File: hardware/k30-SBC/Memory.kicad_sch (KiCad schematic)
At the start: 3 parts, among them U14 AS6C8016, U15 AS6C8016, U16 AM29F040

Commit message: Upgraded project formats to kicad 6.0
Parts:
- U14, U15: symbol ComputieParts:AS6C8016 -> Computie_Memory:AS6C8016
- U16: symbol ComputieParts:AM29F040 -> Computie_Memory:AM29F040
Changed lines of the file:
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@@
     )
   )
-  (symbol (lib_id "ComputieParts:AS6C8016") (at 76.2 58.42 0) (unit 1)
+  (symbol (lib_id "Computie_Memory:AS6C8016") (at 76.2 58.42 0) (unit 1)
     (in_bom yes) (on_board yes)
     (property "Reference" "U14" (id 0) (at 76.2 25.8826 0))
@@
     (pin "9")
   )
-  (symbol (lib_id "ComputieParts:AS6C8016") (at 76.2 138.43 0) (unit 1)
+  (symbol (lib_id "Computie_Memory:AS6C8016") (at 76.2 138.43 0) (unit 1)
     (in_bom yes) (on_board yes)
     (property "Reference" "U15" (id 0) (at 76.2 105.8926 0))
@@
     (pin "1")
   )
-  (symbol (lib_id "ComputieParts:AM29F040") (at 176.53 55.88 0) (unit 1)
+  (symbol (lib_id "Computie_Memory:AM29F040") (at 176.53 55.88 0) (unit 1)
     (in_bom yes) (on_board yes)
     (property "Reference" "U16" (id 0) (at 176.53 25.8826 0))

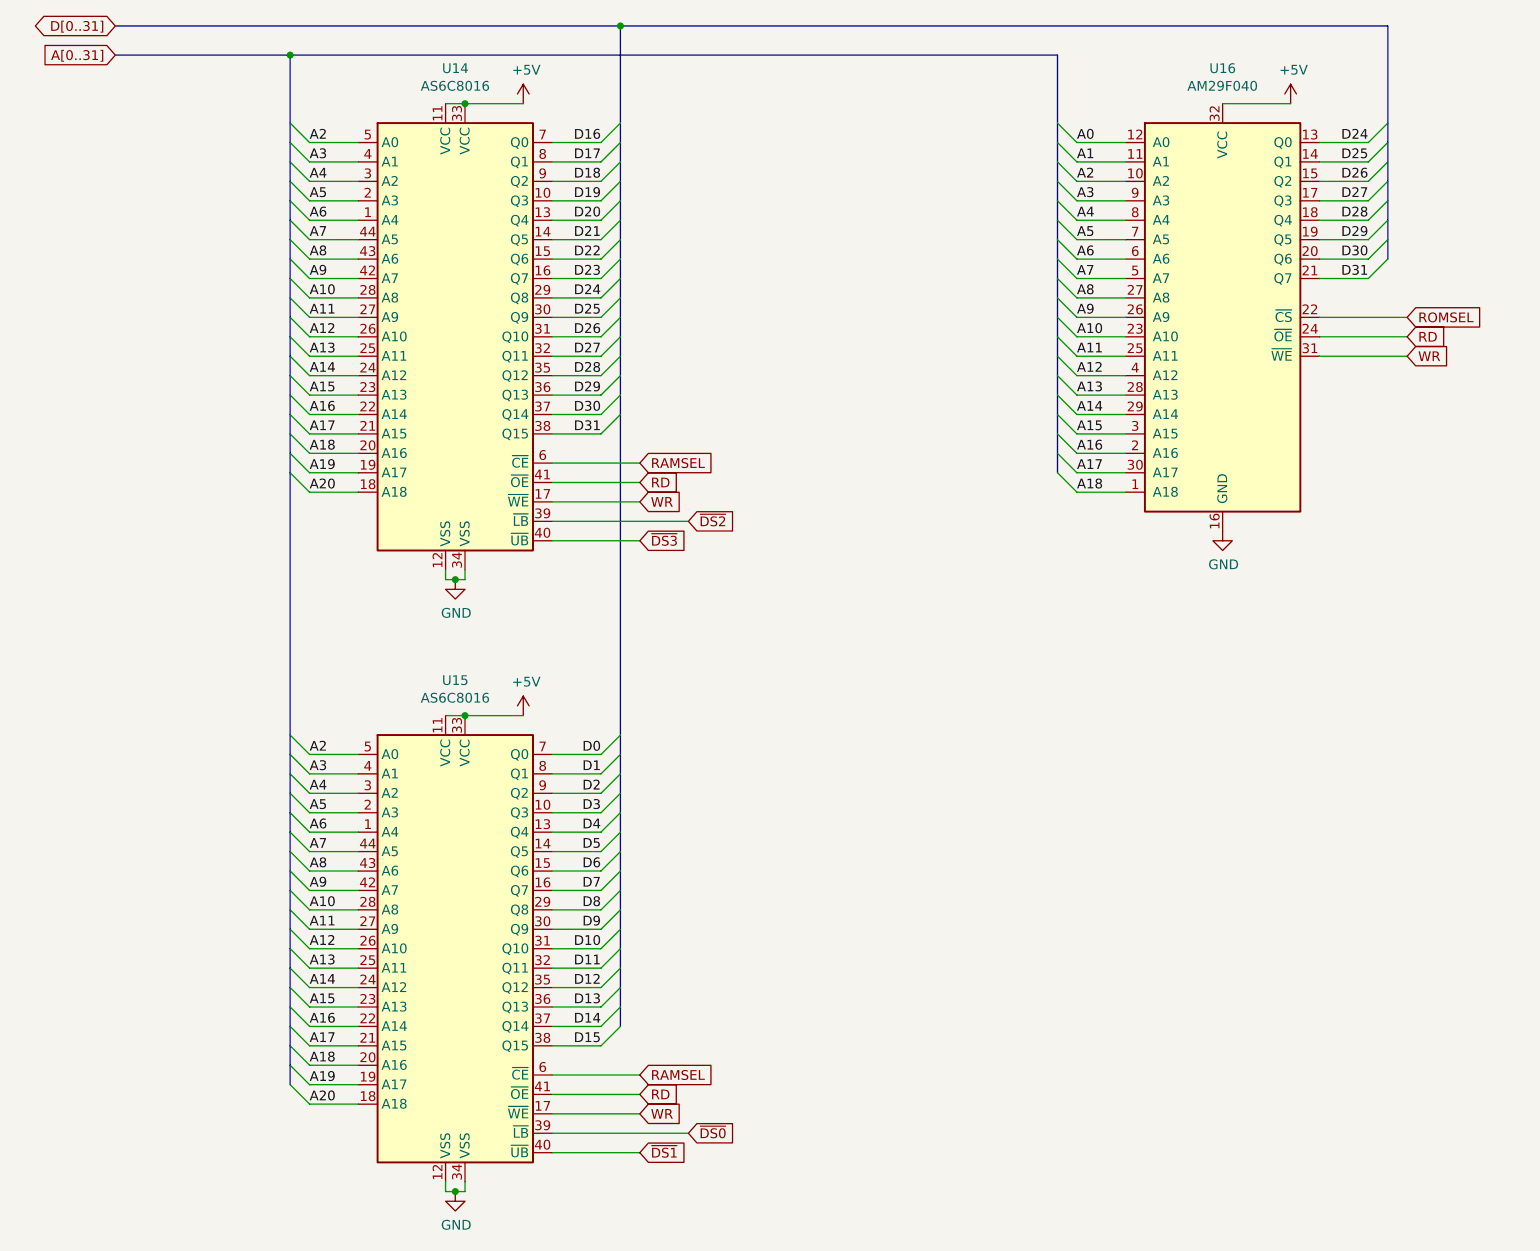
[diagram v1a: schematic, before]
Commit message: Revision 2 of k30-SBC
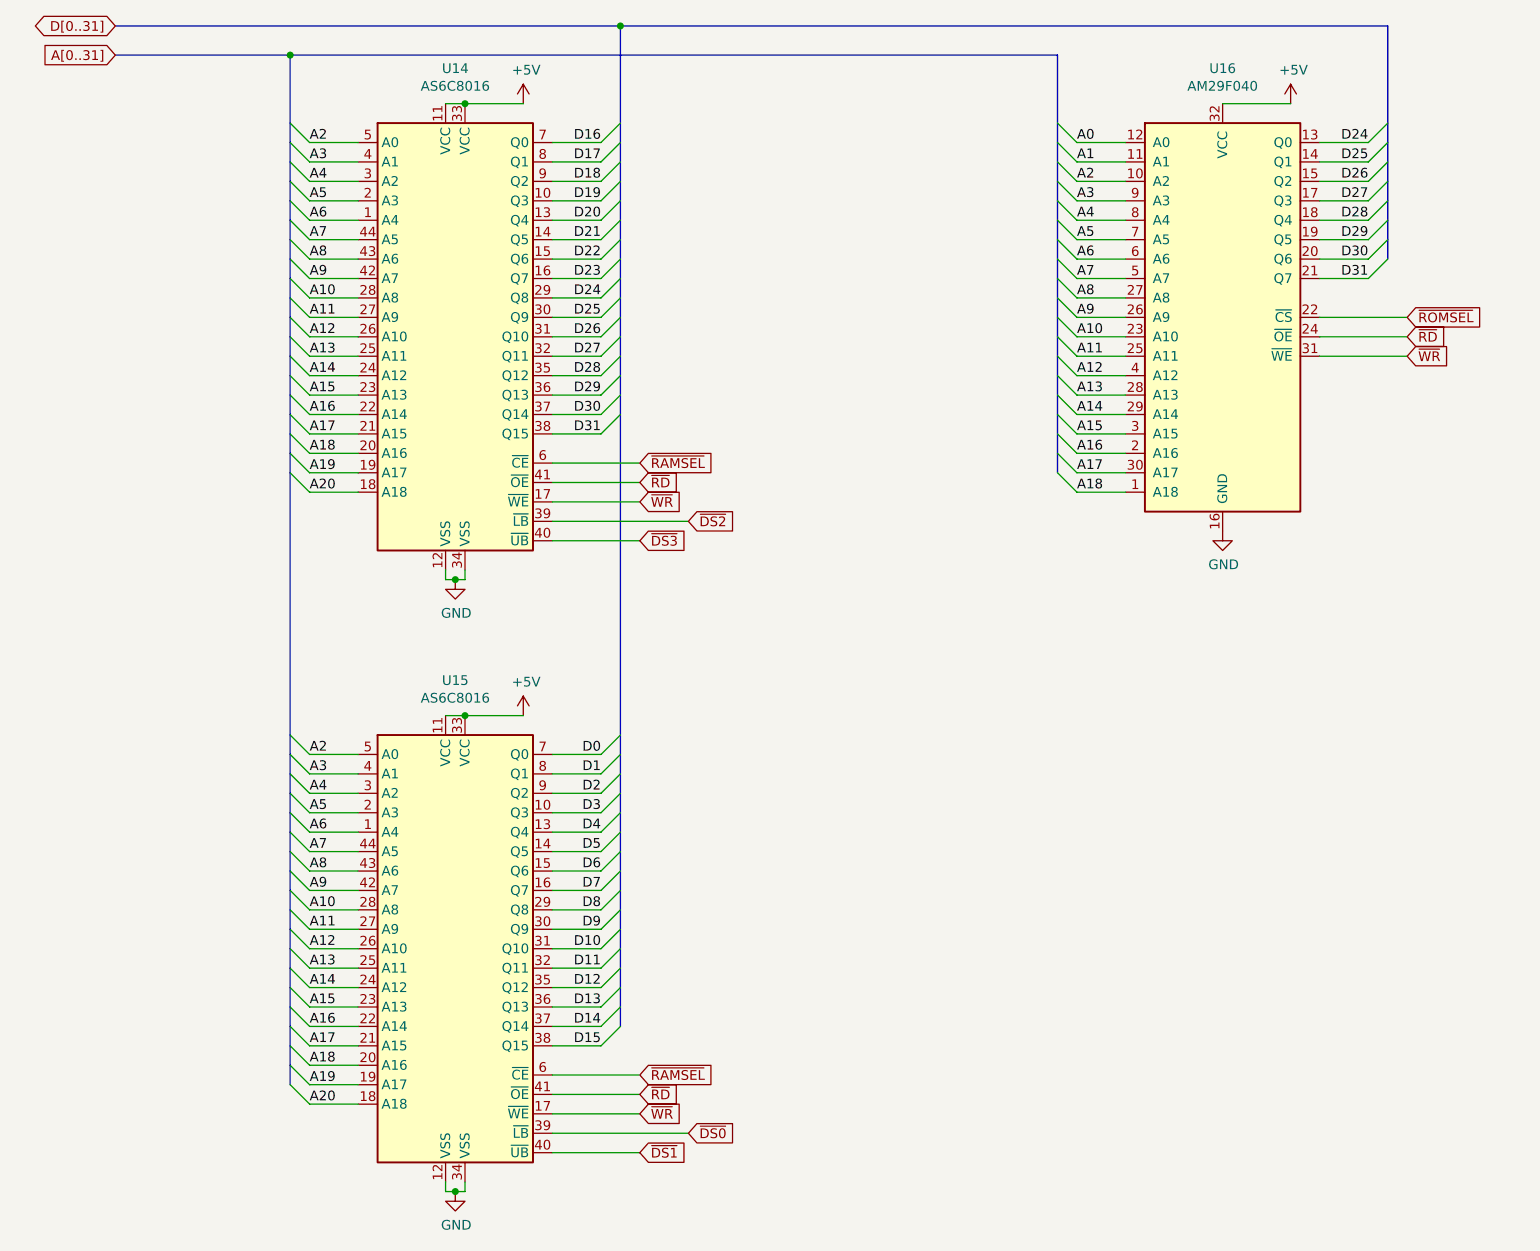
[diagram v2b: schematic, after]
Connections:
- net RAMSEL renamed ~{RAMSEL}
- net RD renamed ~{RD}
- net ROMSEL renamed ~{ROMSEL}
- net WR renamed ~{WR}
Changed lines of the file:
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@@
   (title_block
     (title "k30 SBC")
-    (rev "1")
+    (rev "2")
   )
   (junction (at 77.47 110.49) (diameter 0) (color 0 0 0 0)
@@
     (effects (font (size 1.27 1.27)) (justify left bottom))
   )
-  (global_label "WR" (shape input) (at 100.33 82.55 0) (fields_autoplaced)
+  (global_label "~{WR}" (shape input) (at 100.33 82.55 0) (fields_autoplaced)
     (effects (font (size 1.27 1.27)) (justify left))
     (property "Intersheet References" "${INTERSHEET_REFS}" (id 0) (at 0 0 0)
@@
     )
   )
-  (global_label "WR" (shape input) (at 100.33 162.56 0) (fields_autoplaced)
+  (global_label "~{WR}" (shape input) (at 100.33 162.56 0) (fields_autoplaced)
     (effects (font (size 1.27 1.27)) (justify left))
     (property "Intersheet References" "${INTERSHEET_REFS}" (id 0) (at 0 0 0)
@@
     )
   )
-  (global_label "RD" (shape input) (at 200.66 60.96 0) (fields_autoplaced)
+  (global_label "~{RD}" (shape input) (at 200.66 60.96 0) (fields_autoplaced)
     (effects (font (size 1.27 1.27)) (justify left))
     (property "Intersheet References" "${INTERSHEET_REFS}" (id 0) (at 0 0 0)
@@
     )
   )
-  (global_label "ROMSEL" (shape input) (at 200.66 58.42 0) (fields_autoplaced)
+  (global_label "~{ROMSEL}" (shape input) (at 200.66 58.42 0) (fields_autoplaced)
     (effects (font (size 1.27 1.27)) (justify left))
     (property "Intersheet References" "${INTERSHEET_REFS}" (id 0) (at 0 0 0)
@@
     )
   )
-  (global_label "RAMSEL" (shape input) (at 100.33 157.48 0) (fields_autoplaced)
+  (global_label "~{RAMSEL}" (shape input) (at 100.33 157.48 0) (fields_autoplaced)
     (effects (font (size 1.27 1.27)) (justify left))
     (property "Intersheet References" "${INTERSHEET_REFS}" (id 0) (at 0 0 0)
@@
     )
   )
-  (global_label "RD" (shape input) (at 100.33 160.02 0) (fields_autoplaced)
+  (global_label "~{RD}" (shape input) (at 100.33 160.02 0) (fields_autoplaced)
     (effects (font (size 1.27 1.27)) (justify left))
     (property "Intersheet References" "${INTERSHEET_REFS}" (id 0) (at 0 0 0)
@@
     )
   )
-  (global_label "RAMSEL" (shape input) (at 100.33 77.47 0) (fields_autoplaced)
+  (global_label "~{RAMSEL}" (shape input) (at 100.33 77.47 0) (fields_autoplaced)
     (effects (font (size 1.27 1.27)) (justify left))
     (property "Intersheet References" "${INTERSHEET_REFS}" (id 0) (at 0 0 0)
@@
     )
   )
-  (global_label "RD" (shape input) (at 100.33 80.01 0) (fields_autoplaced)
+  (global_label "~{RD}" (shape input) (at 100.33 80.01 0) (fields_autoplaced)
     (effects (font (size 1.27 1.27)) (justify left))
     (property "Intersheet References" "${INTERSHEET_REFS}" (id 0) (at 0 0 0)
@@
     )
   )
-  (global_label "WR" (shape input) (at 200.66 63.5 0) (fields_autoplaced)
+  (global_label "~{WR}" (shape input) (at 200.66 63.5 0) (fields_autoplaced)
     (effects (font (size 1.27 1.27)) (justify left))
     (property "Intersheet References" "${INTERSHEET_REFS}" (id 0) (at 0 0 0)
